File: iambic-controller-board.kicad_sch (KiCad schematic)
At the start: 16 parts, among them J1 Header 1, J2 AudioJack3, J3 ISP Header, U1 USB_A_PCB, U2 ATtiny85-20S

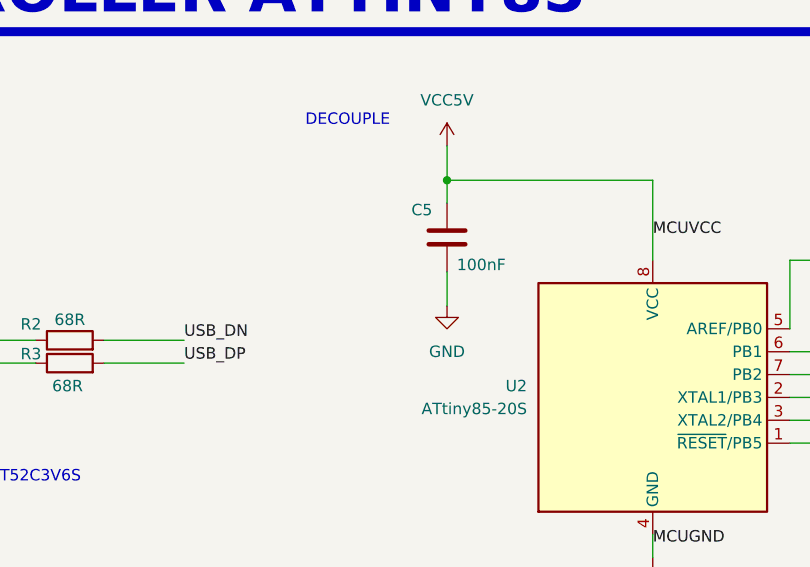
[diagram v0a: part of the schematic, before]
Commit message: final rev1
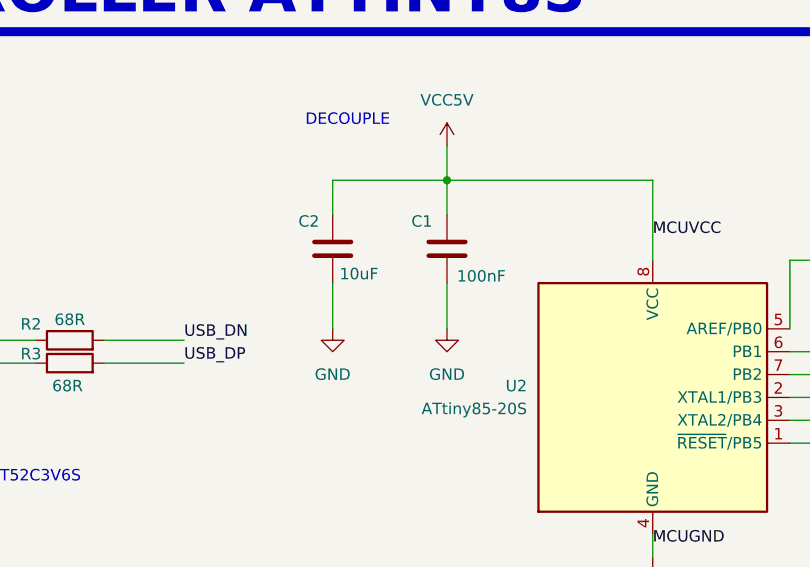
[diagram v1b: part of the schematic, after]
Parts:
- added C2: 10uF, Capacitor_SMD:C_0603_1608Metric, symbol Device:C
- D2, D3: value ~ -> BZT52C3V6S
- U1: footprint Custom_Lib:PCB_USB_connector -> Edge_USB_PCB:PCB_USB_A
- renumbered C5 to C1
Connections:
- net GND: now also C2.2
- net VCC5V: now also C2.1
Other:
- moved on the sheet: C1
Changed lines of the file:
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@@
+	(wire
+		(pts
+			(xy 107.95 41.91) (xy 107.95 45.72)
+		)
+		(stroke
+			(width 0)
+			(type default)
+		)
+	)
 	(wire
 		(pts
@@
 	(wire
 		(pts
+			(xy 120.65 41.91) (xy 120.65 45.72)
+		)
+		(stroke
+			(width 0)
+			(type default)
+		)
+	)
+	(wire
+		(pts
 			(xy 30.48 73.66) (xy 49.53 73.66)
 		)
@@
 	(wire
 		(pts
-			(xy 120.65 41.91) (xy 120.65 44.45)
-		)
-		(stroke
-			(width 0)
-			(type default)
-		)
-	)
-	(wire
-		(pts
 			(xy 176.53 69.85) (xy 187.96 69.85)
 		)
@@
 	(wire
 		(pts
-			(xy 120.65 52.07) (xy 120.65 55.88)
-		)
-		(stroke
-			(width 0)
-			(type default)
-		)
-	)
-	(wire
-		(pts
 			(xy 250.19 62.23) (xy 252.73 62.23)
 		)
@@
 	(wire
 		(pts
+			(xy 120.65 41.91) (xy 107.95 41.91)
+		)
+		(stroke
+			(width 0)
+			(type default)
+		)
+	)
+	(wire
+		(pts
 			(xy 176.53 67.31) (xy 187.96 67.31)
 		)
@@
 	(wire
 		(pts
+			(xy 107.95 53.34) (xy 107.95 58.42)
+		)
+		(stroke
+			(width 0)
+			(type default)
+		)
+	)
+	(wire
+		(pts
 			(xy 143.51 41.91) (xy 143.51 50.8)
 		)
@@
 		(pts
 			(xy 143.51 81.28) (xy 143.51 83.82)
+		)
+		(stroke
+			(width 0)
+			(type default)
+		)
+	)
+	(wire
+		(pts
+			(xy 120.65 53.34) (xy 120.65 58.42)
 		)
 		(stroke
@@
 	(symbol
 		(lib_id "Device:C")
-		(at 120.65 48.26 180)
+		(at 120.65 49.53 180)
 		(unit 1)
 		(exclude_from_sim no)
@@
 		(on_board yes)
 		(dnp no)
-		(property "Reference" "C5"
-			(at 117.856 45.212 0)
+		(property "Reference" "C1"
+			(at 117.856 46.482 0)
 			(effects
 				(font
@@
 		)
 		(property "Value" "100nF"
-			(at 124.46 51.308 0)
+			(at 124.46 52.578 0)
 			(effects
 				(font
@@
 		)
 		(property "Footprint" "Capacitor_SMD:C_0603_1608Metric"
-			(at 119.6848 44.45 0)
+			(at 119.6848 45.72 0)
 			(effects
 				(font
@@
 		)
 		(property "Datasheet" "~"
-			(at 120.65 48.26 0)
+			(at 120.65 49.53 0)
 			(effects
 				(font
@@
 		)
 		(property "Description" "Unpolarized capacitor"
-			(at 120.65 48.26 0)
+			(at 120.65 49.53 0)
 			(effects
 				(font
@@
 		)
 		(property "Untitled Field" ""
-			(at 120.65 48.26 0)
+			(at 120.65 49.53 0)
 			(effects
 				(font
@@
 			(project "iambic-controller-board"
 				(path "/cbe024e5-cc72-4953-a772-8be6edb02bba"
-					(reference "C5")
+					(reference "C1")
 					(unit 1)
 				)
@@
 	)
 	(symbol
+		(lib_id "power:GND")
+		(at 107.95 58.42 0)
+		(unit 1)
+		(exclude_from_sim no)
+		(in_bom yes)
+		(on_board yes)
+		(dnp no)
+		(fields_autoplaced yes)
+		(property "Reference" "#PWR02"
+			(at 107.95 64.77 0)
+			(effects
+				(font
+					(size 1.27 1.27)
+				)
+				(hide yes)
+			)
+		)
+		(property "Value" "GND"
+			(at 107.95 63.5 0)
+			(effects
+				(font
+					(size 1.27 1.27)
+				)
+			)
+		)
+		(property "Footprint" ""
+			(at 107.95 58.42 0)
+			(effects
+				(font
+					(size 1.27 1.27)
+				)
+				(hide yes)
+			)
+		)
+		(property "Datasheet" ""
+			(at 107.95 58.42 0)
+			(effects
+				(font
+					(size 1.27 1.27)
+				)
+				(hide yes)
+			)
+		)
+		(property "Description" "Power symbol creates a global label with name \"GND\" , ground"
+			(at 107.95 58.42 0)
+			(effects
+				(font
+					(size 1.27 1.27)
+				)
+				(hide yes)
+			)
+		)
+		(pin "1"
+		)
+		(instances
+			(project "iambic-controller-board"
+				(path "/cbe024e5-cc72-4953-a772-8be6edb02bba"
+					(reference "#PWR02")
+					(unit 1)
+				)
+			)
+		)
+	)
+	(symbol
+		(lib_id "Device:C")
+		(at 107.95 49.53 0)
+		(unit 1)
+		(exclude_from_sim no)
+		(in_bom yes)
+		(on_board yes)
+		(dnp no)
+		(property "Reference" "C2"
+			(at 104.14 46.482 0)
+			(effects
+				(font
+					(size 1.27 1.27)
+				)
+				(justify left)
+			)
+		)
+		(property "Value" "10uF"
+			(at 108.712 52.324 0)
+			(effects
+				(font
+					(size 1.27 1.27)
+				)
+				(justify left)
+			)
+		)
+		(property "Footprint" "Capacitor_SMD:C_0603_1608Metric"
+			(at 108.9152 53.34 0)
+			(effects
+				(font
+					(size 1.27 1.27)
+				)
+				(hide yes)
+			)
+		)
+		(property "Datasheet" "~"
+			(at 107.95 49.53 0)
+			(effects
+				(font
+					(size 1.27 1.27)
+				)
+				(hide yes)
+			)
+		)
+		(property "Description" "Unpolarized capacitor"
+			(at 107.95 49.53 0)
+			(effects
+				(font
+					(size 1.27 1.27)
+				)
+				(hide yes)
+			)
+		)
+		(property "Untitled Field" ""
+			(at 107.95 49.53 0)
+			(effects
+				(font
+					(size 1.27 1.27)
+				)
+				(hide yes)
+			)
+		)
+		(pin "2"
+		)
+		(pin "1"
+		)
+		(instances
+			(project "iambic-controller-board"
+				(path "/cbe024e5-cc72-4953-a772-8be6edb02bba"
+					(reference "C2")
+					(unit 1)
+				)
+			)
+		)
+	)
+	(symbol
 		(lib_id "Connector:USB_A")
 		(at 30.48 59.69 0)
@@
 			)
 		)
-		(property "Footprint" "Custom_Lib:PCB_USB_connector"
+		(property "Footprint" "Edge_USB_PCB:PCB_USB_A"
 			(at 34.29 60.96 0)
 			(effects
@@
 	(symbol
 		(lib_id "power:GND")
-		(at 120.65 55.88 0)
+		(at 120.65 58.42 0)
 		(unit 1)
 		(exclude_from_sim no)
@@
 		(fields_autoplaced yes)
 		(property "Reference" "#PWR013"
-			(at 120.65 62.23 0)
+			(at 120.65 64.77 0)
 			(effects
 				(font
@@
 		)
 		(property "Value" "GND"
-			(at 120.65 60.96 0)
+			(at 120.65 63.5 0)
 			(effects
 				(font
@@
 		)
 		(property "Footprint" ""
-			(at 120.65 55.88 0)
+			(at 120.65 58.42 0)
 			(effects
 				(font
@@
 		)
 		(property "Datasheet" ""
-			(at 120.65 55.88 0)
+			(at 120.65 58.42 0)
 			(effects
 				(font
@@
 		)
 		(property "Description" "Power symbol creates a global label with name \"GND\" , ground"
-			(at 120.65 55.88 0)
+			(at 120.65 58.42 0)
 			(effects
 				(font
@@
 			)
 		)
-		(property "Value" "~"
+		(property "Value" "BZT52C3V6S"
 			(at 56.134 78.232 90)
 			(effects
@@
 		)
 		(property "Description" "Zener diode"
+			(at 57.15 71.12 0)
+			(effects
+				(font
+					(size 1.27 1.27)
+				)
+				(hide yes)
+			)
+		)
+		(property "Untitled Field" ""
 			(at 57.15 71.12 0)
 			(effects
@@
 			)
 		)
-		(property "Value" "~"
+		(property "Value" "BZT52C3V6S"
 			(at 82.55 74.93 90)
 			(effects
@@
 			(at 66.04 71.12 0)
 			(effects
+				(font
+					(size 1.27 1.27)
+				)
+				(hide yes)
+			)
+		)
+		(property "Untitled Field" ""
+			(at 66.04 71.12 0)
+			(effects

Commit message: Fixed weird footprints
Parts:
- D1: footprint Diode_SMD:D_0201_0603Metric -> Diode_SMD:D_SOD-123
- D2, D3: value BZT52C3V6S -> 3V6; footprint Diode_SMD:D_0201_0603Metric -> Diode_SMD:D_SOD-323
- D4, D5: footprint LED_SMD:LED_0201_0603Metric -> LED_SMD:LED_0603_1608Metric
- R1, R2, R3, R4, R5: footprint Resistor_SMD:R_0201_0603Metric -> Resistor_SMD:R_0603_1608Metric
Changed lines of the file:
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@@
 			)
 		)
-		(property "Footprint" "LED_SMD:LED_0201_0603Metric"
+		(property "Footprint" "LED_SMD:LED_0603_1608Metric"
 			(at 107.95 138.43 0)
 			(effects
@@
 			)
 		)
-		(property "Footprint" "Resistor_SMD:R_0201_0603Metric"
+		(property "Footprint" "Resistor_SMD:R_0603_1608Metric"
 			(at 106.172 152.4 90)
 			(effects
@@
 			)
 		)
-		(property "Footprint" "Diode_SMD:D_0201_0603Metric"
+		(property "Footprint" "Diode_SMD:D_SOD-123"
 			(at 40.64 48.26 0)
 			(effects
@@
 		)
 		(property "Description" "Schottky diode"
+			(at 40.64 48.26 0)
+			(effects
+				(font
+					(size 1.27 1.27)
+				)
+				(hide yes)
+			)
+		)
+		(property "Untitled Field" ""
 			(at 40.64 48.26 0)
 			(effects
@@
 			)
 		)
-		(property "Footprint" "Resistor_SMD:R_0201_0603Metric"
+		(property "Footprint" "Resistor_SMD:R_0603_1608Metric"
 			(at 55.372 48.26 90)
 			(effects
@@
 			)
 		)
-		(property "Footprint" "Resistor_SMD:R_0201_0603Metric"
+		(property "Footprint" "Resistor_SMD:R_0603_1608Metric"
 			(at 126.492 152.4 90)
 			(effects
@@
 			)
 		)
-		(property "Value" "BZT52C3V6S"
+		(property "Value" "3V6"
 			(at 56.134 78.232 90)
 			(effects
@@
 			)
 		)
-		(property "Footprint" "Diode_SMD:D_0201_0603Metric"
+		(property "Footprint" "Diode_SMD:D_SOD-323"
 			(at 57.15 71.12 0)
 			(effects
@@
 			)
 		)
-		(property "Footprint" "Resistor_SMD:R_0201_0603Metric"
+		(property "Footprint" "Resistor_SMD:R_0603_1608Metric"
 			(at 78.74 61.468 90)
 			(effects
@@
 		)
 		(property "Description" "Resistor"
+			(at 78.74 59.69 0)
+			(effects
+				(font
+					(size 1.27 1.27)
+				)
+				(hide yes)
+			)
+		)
+		(property "Untitled Field" ""
 			(at 78.74 59.69 0)
 			(effects
@@
 			)
 		)
-		(property "Value" "BZT52C3V6S"
+		(property "Value" "3V6"
 			(at 82.55 74.93 90)
 			(effects
@@
 			)
 		)
-		(property "Footprint" "Diode_SMD:D_0201_0603Metric"
+		(property "Footprint" "Diode_SMD:D_SOD-323"
 			(at 66.04 71.12 0)
 			(effects
@@
 			)
 		)
-		(property "Footprint" "LED_SMD:LED_0201_0603Metric"
+		(property "Footprint" "LED_SMD:LED_0603_1608Metric"
 			(at 128.27 138.43 0)
 			(effects
@@
 			)
 		)
-		(property "Footprint" "Resistor_SMD:R_0201_0603Metric"
+		(property "Footprint" "Resistor_SMD:R_0603_1608Metric"
 			(at 78.74 64.008 90)
 			(effects
@@
 			(at 78.74 62.23 0)
 			(effects
+				(font
+					(size 1.27 1.27)
+				)
+				(hide yes)
+			)
+		)
+		(property "Untitled Field" ""
+			(at 78.74 62.23 0)
+			(effects
